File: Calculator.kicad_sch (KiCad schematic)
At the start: 2 parts, among them U1 RP2040

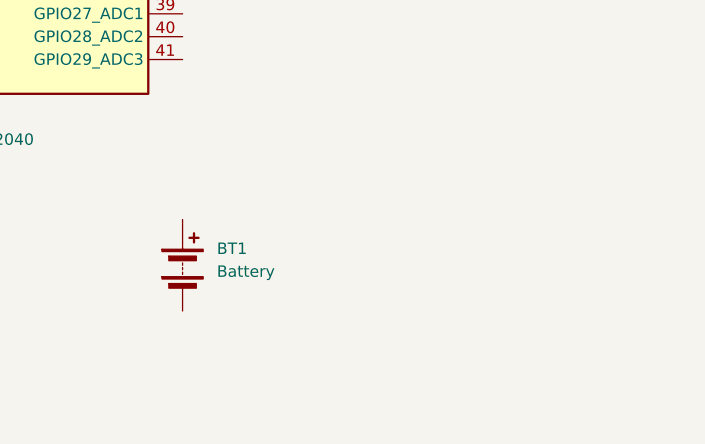
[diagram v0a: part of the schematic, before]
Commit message: progress
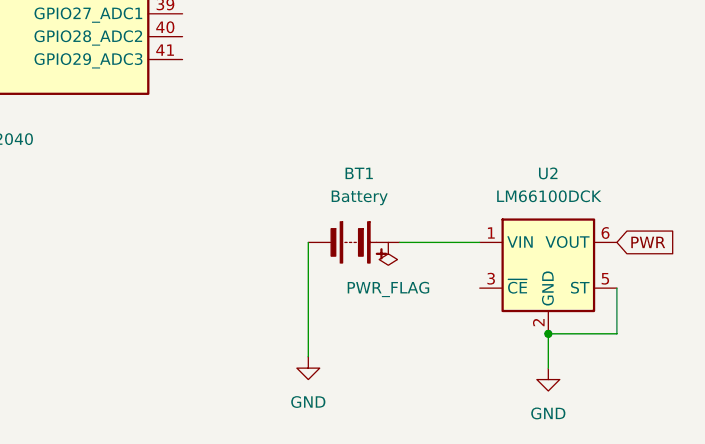
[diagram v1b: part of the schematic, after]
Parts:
- added U2: LM66100DCK, Package_TO_SOT_SMD:SOT-363_SC-70-6, symbol Power_Management:LM66100DCK
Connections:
- net at BT1.1 (+): now also U2.1 (VIN)
- net GND: now reaches BT1.2 (-)
- net GND: now also U2.2 (GND), U2.5 (ST)
- new net PWR: U2.6 (VOUT)
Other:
- moved on the sheet: BT1
